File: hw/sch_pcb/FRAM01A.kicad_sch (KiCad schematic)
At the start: 8 parts, among them IC1 CY15B108QN-40SXI, J1 HEADER_2x03_PARALLEL, J2 HEADER_2x04

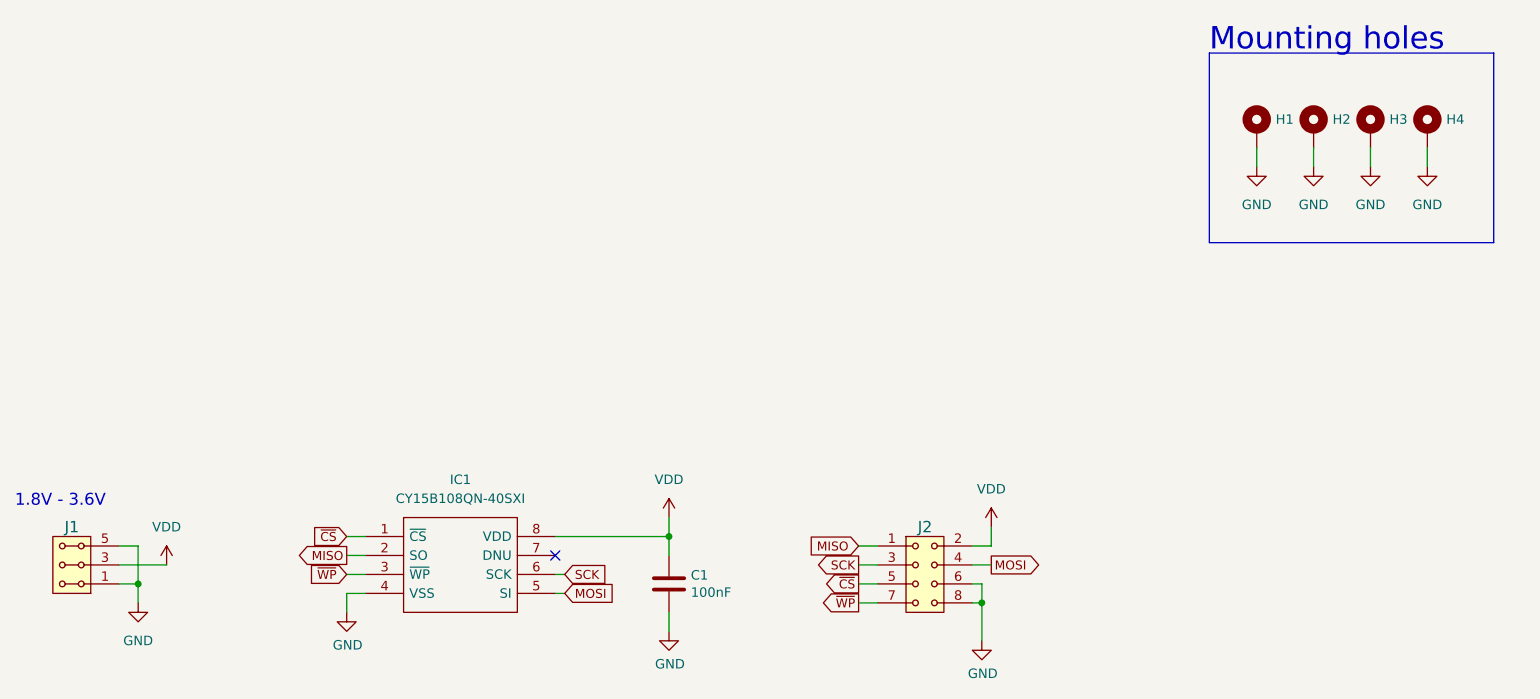
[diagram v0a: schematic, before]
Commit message: pcb layout update, ready for check
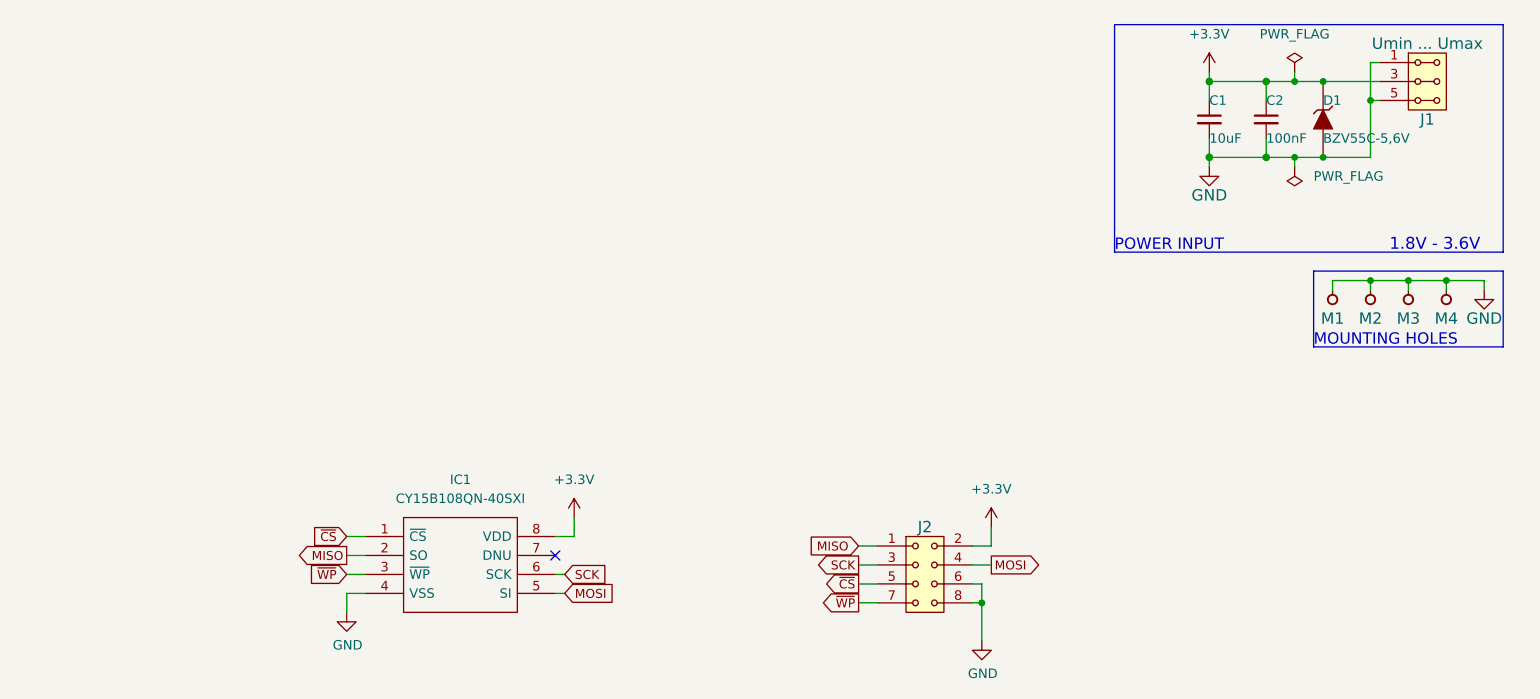
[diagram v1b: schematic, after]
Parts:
- removed C1: 100nF, Mlab_R:SMD-0805, symbol DATALOGGER01A-rescue:C-device
- removed H1, H2, H3, H4: MountingHole_Pad, Mlab_Mechanical:MountingHole_3mm, symbol Mechanical:MountingHole_Pad
- removed J1: HEADER_2x03_PARALLEL, Mlab_Pin_Headers:Straight_2x03, symbol MLAB_HEADER:HEADER_2x03_PARALLEL
- added C1: 10uF, Capacitor_SMD:C_0805_2012Metric, symbol ISM02A-rescue:C_Small-Device-ISM02A-rescue
- added C2: 100nF, Capacitor_SMD:C_0805_2012Metric, symbol ISM02A-rescue:C_Small-Device-ISM02A-rescue
- added D1: BZV55C-5,6V, Diode_SMD:D_SMA, symbol ISM02A-rescue:D_ZENER-MLAB_D
- added J1: Umin ... Umax, Mlab_Pin_Headers:Straight_2x03, symbol header:HEADER_2x03_PARALLEL
- added M1, M2: HOLE M3, Mlab_Mechanical:MountingHole_3mm, symbol mlab-default-rescue:HOLE
- added M3, M4: HOLE, Mlab_Mechanical:MountingHole_3mm, symbol mlab-default-rescue:HOLE
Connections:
- net GND: now also C1.2, C2.2, D1.2 (A), J1.1, J1.2, J1.5, J1.6, M1.1, M2.1, M3.1, M4.1
- net VDD renamed +3.3V
- net +3.3V: now also C1.1, C2.1, D1.1 (K), J1.3, J1.4
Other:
- note added: "MOUNTING HOLES"
- note added: "POWER INPUT"
- note removed: "Mounting holes"
